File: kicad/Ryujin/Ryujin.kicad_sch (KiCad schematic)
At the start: 21 parts, among them J1 BAT, J2 SDI12, Q1 IRLML6244, U1 TXS0101DBV, U2 R-78E5.0-0.5, U3 W25Q32JVSS, U4 SHTC3

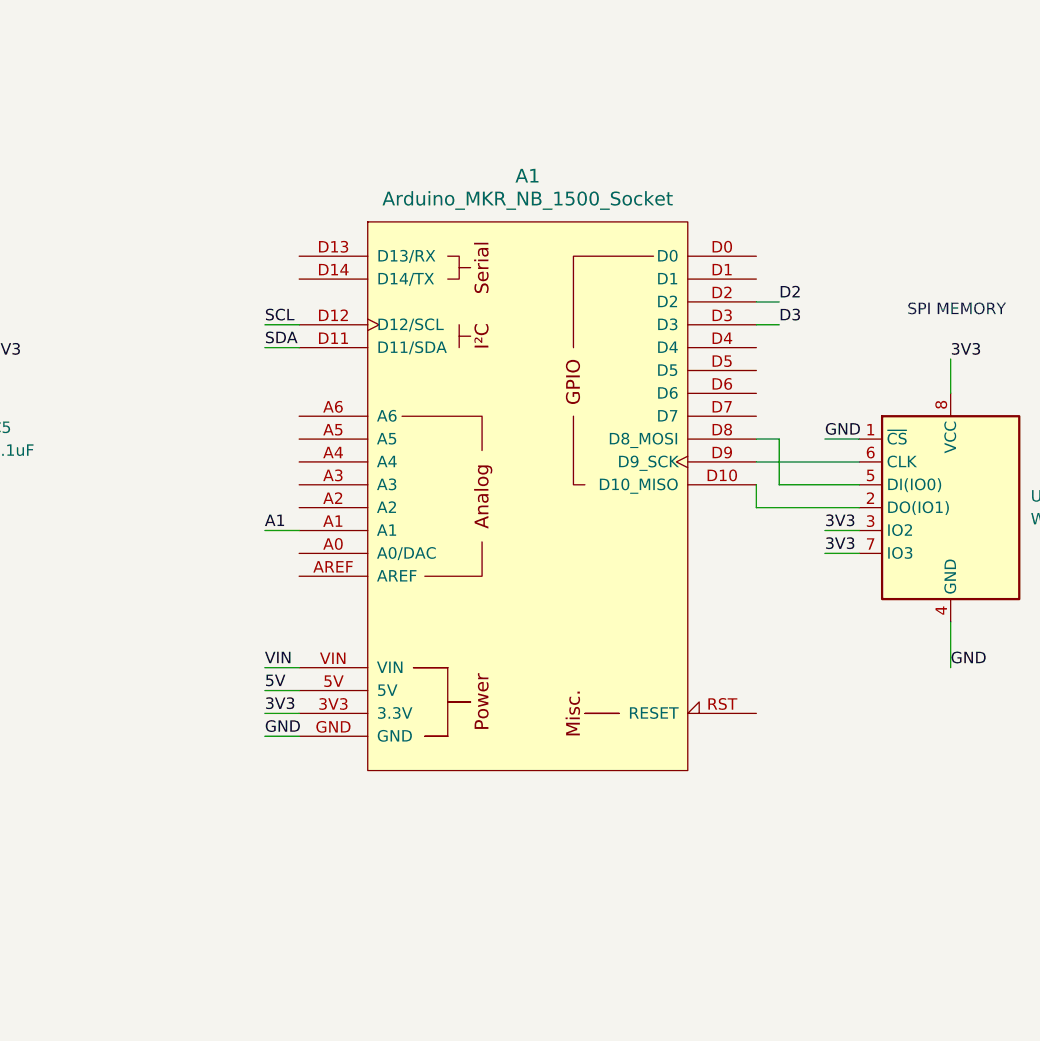
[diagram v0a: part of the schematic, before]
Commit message: Gladiator
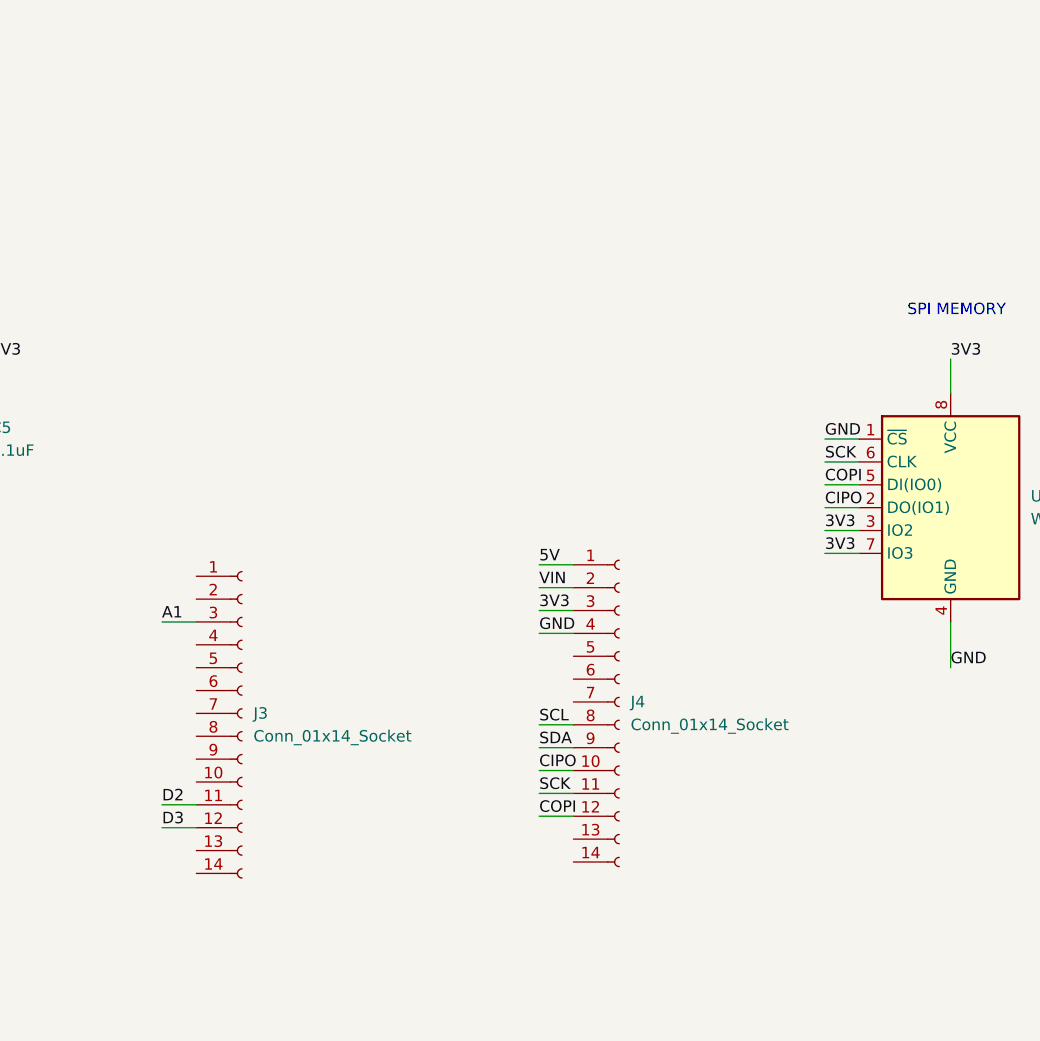
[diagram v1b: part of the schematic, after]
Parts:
- removed A1: Arduino_MKR_NB_1500_Socket, Custom:Arduino_MKR_NB_1500_Socket, symbol PCM_arduino-library:Arduino_MKR_NB_1500_Socket
- added J3, J4: Conn_01x14_Socket, Custom:65342372, symbol Connector:Conn_01x14_Socket
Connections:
- net 3V3: now also J4.3 (Pin_3)
- net 5V: now also J4.1 (Pin_1)
- net A1: now also J3.3 (Pin_3)
- net D2: now also J3.11 (Pin_11)
- net D3: now also J3.12 (Pin_12)
- net GND: now also J4.4 (Pin_4)
- net SCL: now also J4.8 (Pin_8)
- net SDA: now also J4.9 (Pin_9)
- net VIN: now also J4.2 (Pin_2)
- net CIPO: now reaches U3.2 (DO(IO1))
- net CIPO: now also J4.10 (Pin_10)
- net COPI: now reaches U3.5 (DI(IO0))
- net COPI: now also J4.12 (Pin_12)
- net SCK: now reaches U3.6 (CLK)
- net SCK: now also J4.11 (Pin_11)
